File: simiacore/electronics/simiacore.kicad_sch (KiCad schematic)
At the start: 31 parts, among them J1 X_STEP_DRIVER, J10 Y1_LIM_PORT, J2 Y0_STEP_DRIVER, J3 Z_STEP_DRIVER, J4 Y1_STEP_DRIVER, J5 X_STEP, J6 X_LIM_PORT, J6 Y0_STEP, J7 Y0_LIM_PORT, J7 Z_STEP, J8 Y1_STEP, J8 Z_LIM_PORT, J9 SPINDLE_SPEED, SW1 LOGIC_TOGGLE, SW2 LOGIC_TOGGLE, SW3 LOGIC_TOGGLE, SW4 LOGIC_TOGGLE, U1 NCV20231XV53T2G, U3 PicoW

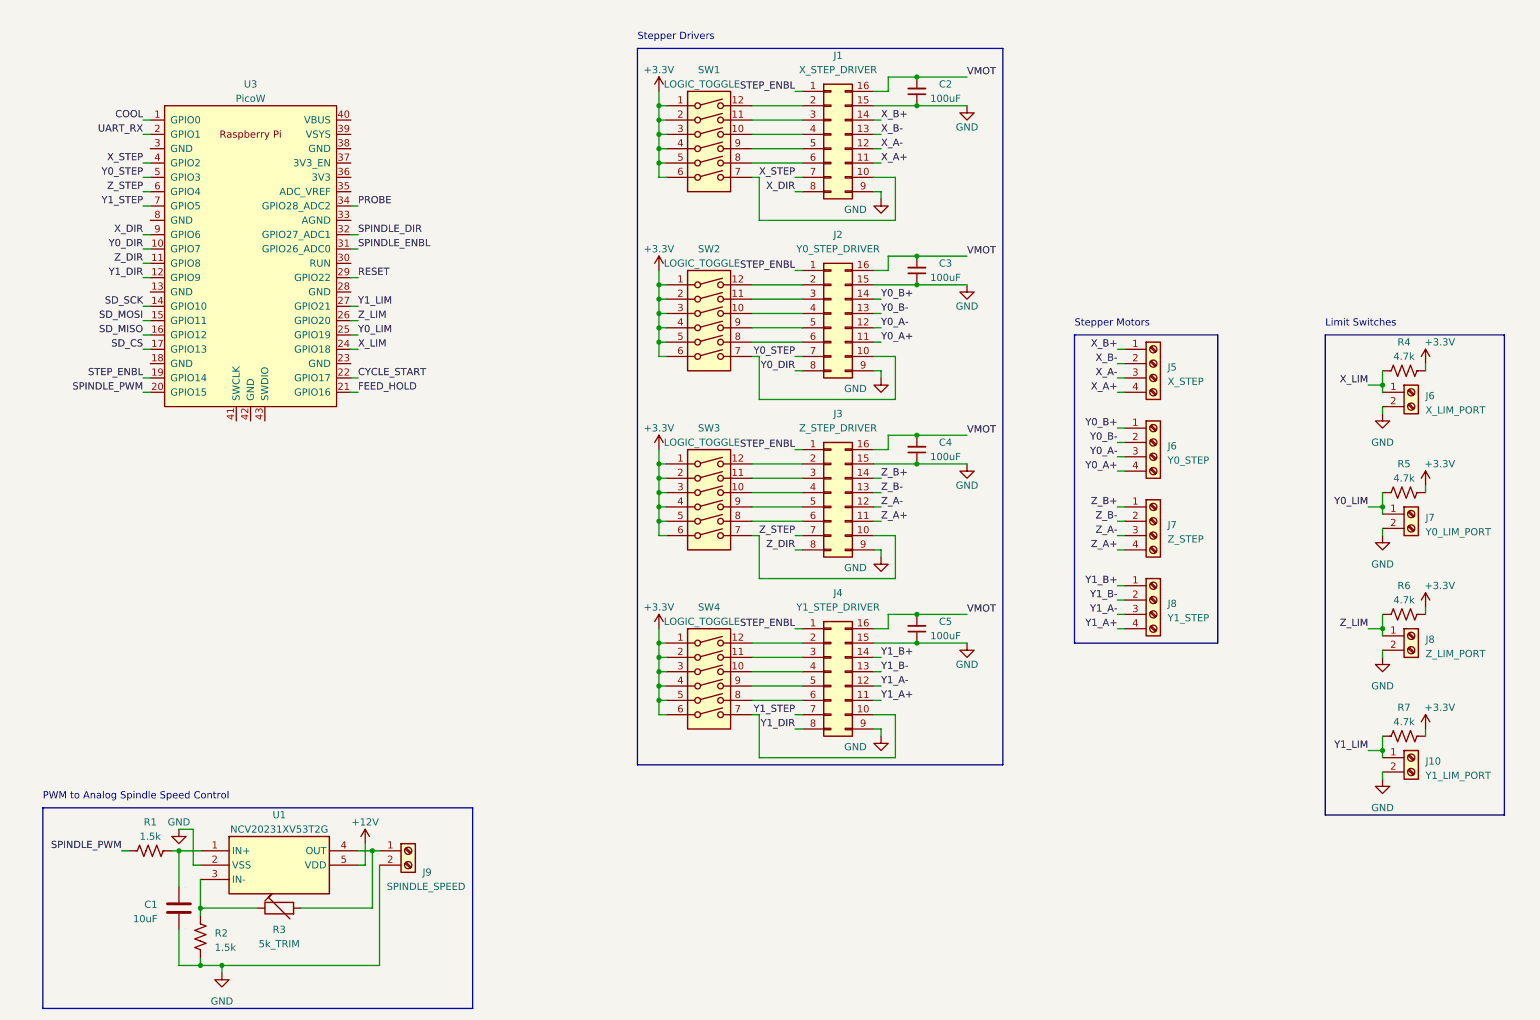
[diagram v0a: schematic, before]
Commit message: did some work
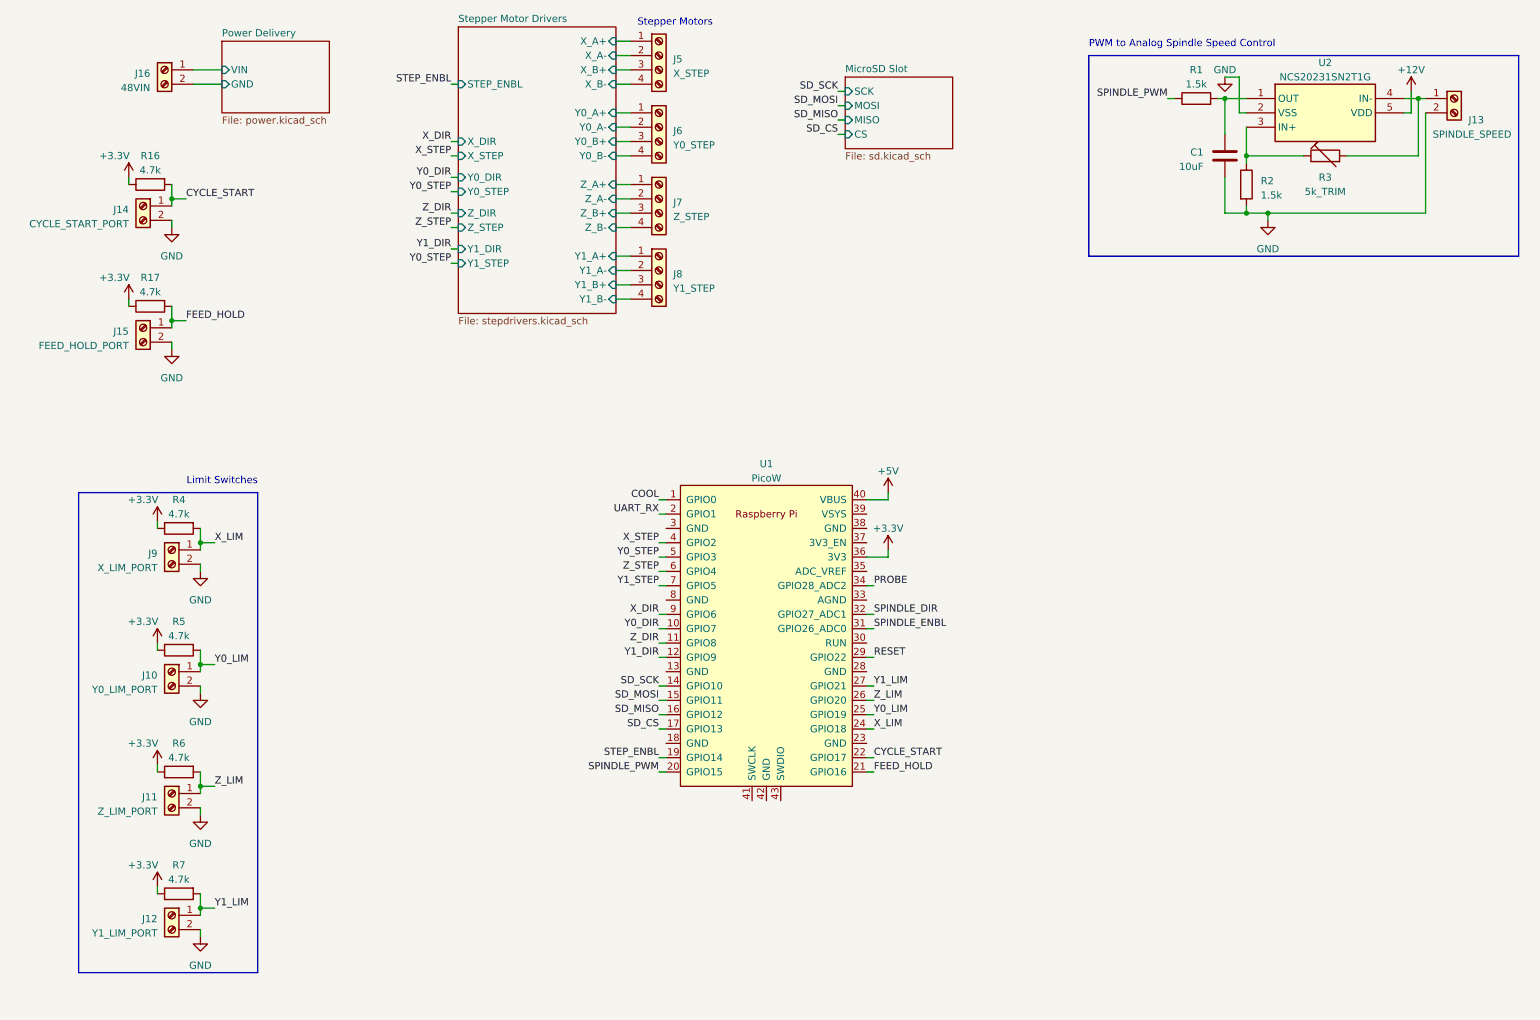
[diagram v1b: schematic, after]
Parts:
- removed C2, C3, C4, C5: 100uF, mainboardlibrary:MAL203859101E3, symbol Device:C_Small
- removed J1: X_STEP_DRIVER, mainboardlibrary:16pinStepperDriverHeader, symbol Connector_Generic:Conn_02x08_Counter_Clockwise
- removed J2: Y0_STEP_DRIVER, mainboardlibrary:16pinStepperDriverHeader, symbol Connector_Generic:Conn_02x08_Counter_Clockwise
- removed J3: Z_STEP_DRIVER, mainboardlibrary:16pinStepperDriverHeader, symbol Connector_Generic:Conn_02x08_Counter_Clockwise
- removed J4: Y1_STEP_DRIVER, mainboardlibrary:16pinStepperDriverHeader, symbol Connector_Generic:Conn_02x08_Counter_Clockwise
- removed SW1, SW2, SW3, SW4: LOGIC_TOGGLE, mainboardlibrary:CFS-0600TB, symbol Switch:SW_DIP_x06
- removed U1: NCV20231XV53T2G, SOTFL50P160X60-5N, symbol SamacSys_Parts:NCV20231XV53T2G
- added J14: CYCLE_START_PORT, SamacSys_Parts:1190297, symbol Connector:Screw_Terminal_01x02
- added J15: FEED_HOLD_PORT, SamacSys_Parts:1190297, symbol Connector:Screw_Terminal_01x02
- added J16: 48VIN, SamacSys_Parts:1190297, symbol Connector:Screw_Terminal_01x02
- added R16, R17: 4.7k, SamacSys_Parts:RESC6432X65N, symbol Device:R
- added U2: NCS20231SN2T1G, SOT95P275X110-5N, symbol SamacSys_Parts:NCS20231SN2T1G
- J5, J6, J7, J8: footprint mainboardlibrary:1190299 -> SamacSys_Parts:1190299
- R1, R2, R4, R5, R6, R7: symbol Device:R_US -> Device:R
- U1: renamed from U3; footprint RPi_PicoW:RPi_Pico_SMD_TH -> RPi_Pico:RPi_PicoW_SMD_TH
- renumbered J7 to J10, J8 to J11, J10 to J12, J9 to J13, J6 to J9
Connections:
- net +12V: now also U2.5 (VDD)
- net +3.3V: now also U1.36 (3V3), R16.1, R17.1
- net CYCLE_START: now also J14.1 (Pin_1), R16.2
- net FEED_HOLD: now also J15.1 (Pin_1), R17.2
- net GND: now also J14.2 (Pin_2), J15.2 (Pin_2), U2.2 (VSS)
- net at R2.1, R3.1: now also U2.3 (IN+)
- net at C1.1, R1.2: now also U2.1 (OUT)
- net at J13.1 (Pin_1), R3.2: now also U2.4 (IN-)
- net +5V: now reaches U1.40 (VBUS)
- net X_A+ renamed Stepper Motor Drivers/X_B-
- net X_A- renamed Stepper Motor Drivers/X_B+
- net X_B+ renamed Stepper Motor Drivers/X_A+
- net X_B- renamed Stepper Motor Drivers/X_A-
- net Y0_A+ renamed Stepper Motor Drivers/Y0_B-
- net Y0_A- renamed Stepper Motor Drivers/Y0_B+
- net Y0_B+ renamed Stepper Motor Drivers/Y0_A+
- net Y0_B- renamed Stepper Motor Drivers/Y0_A-
- net Y1_A+ renamed Stepper Motor Drivers/Y1_B-
- net Y1_A- renamed Stepper Motor Drivers/Y1_B+
- net Y1_B+ renamed Stepper Motor Drivers/Y1_A+
- net Y1_B- renamed Stepper Motor Drivers/Y1_A-
- net Z_A+ renamed Stepper Motor Drivers/Z_B-
- net Z_A- renamed Stepper Motor Drivers/Z_B+
- net Z_B+ renamed Stepper Motor Drivers/Z_A+
- net Z_B- renamed Stepper Motor Drivers/Z_A-
- new net Power Delivery/GND: J16.2 (Pin_2)
- new net Power Delivery/VIN: J16.1 (Pin_1)
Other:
- added sheet MicroSD Slot (sd.kicad_sch)
- added sheet Power Delivery (power.kicad_sch)
- added sheet Stepper Motor Drivers (stepdrivers.kicad_sch)
- note removed: "Stepper Drivers"
- moved on the sheet: C1, J10, J11, J12, J13, J5, J6, J7, J8, J9, R3, U1
